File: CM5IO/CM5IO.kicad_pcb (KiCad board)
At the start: 4 copper layers, 59.7 x 78 mm, 64 parts, among them J1 POWER TERMINAL, J11 USB_C_Receptacle_USB2.0, J12 USB3_A, J14 JST_SHBM04B-SRSS-TB, J16 Conn_01x22_Female, J2 Conn_02x06_Odd_Even, J22 46765-1301, J4 J_PSU_EN, J5 Conn_01x22_Female, J7 Micro_SD_Card_Det, J8 THD-20-R, SW1 Right angle Tact button, U12 RT9742SNGV, U18 RT9742GGJ5, U6 AP22653W6

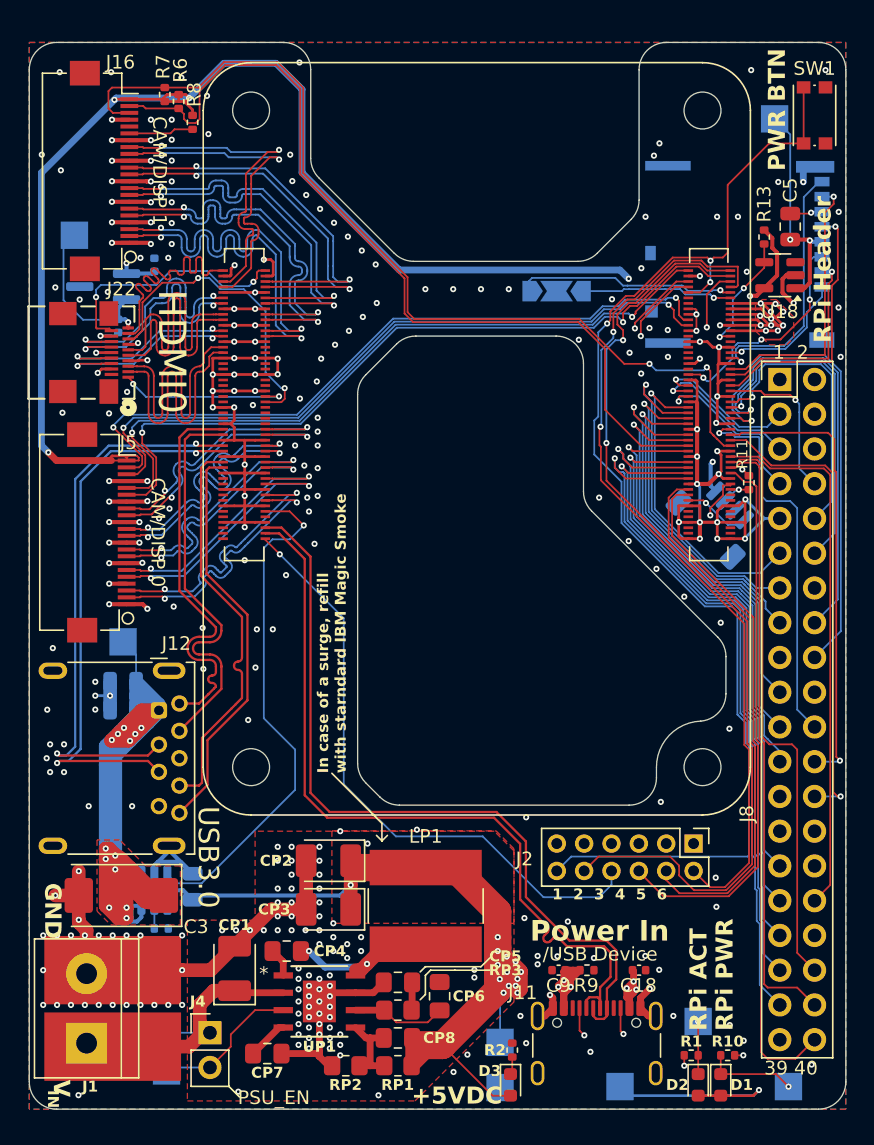
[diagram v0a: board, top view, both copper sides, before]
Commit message: final changes before ordering the design
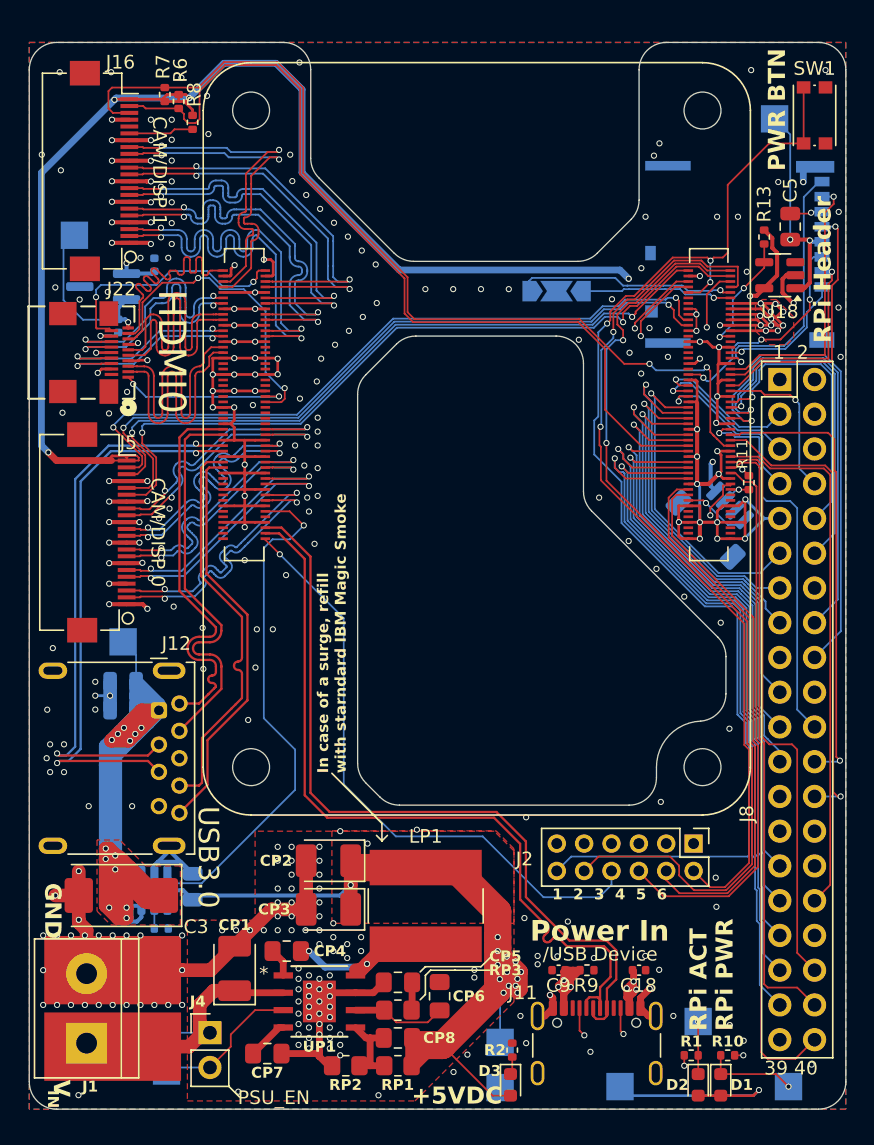
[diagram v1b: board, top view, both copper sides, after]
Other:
- board text added: "100R"
- board text added: "90R"
